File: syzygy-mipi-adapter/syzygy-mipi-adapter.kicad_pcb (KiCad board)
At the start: 4 copper layers, 45 x 70 mm, 67 parts, among them J1 Conn_02x06_Odd_Even, J10 501951-2230, J2 SYZYGY_STD, J3 Conn_01x02, J5 SM03B-SRSS-TB, J8 501951-2230, J9 501951-2230, Q1 DMG1024UV-7, Q2 DMG1024UV-7, U1 RP2350_80QFN, U10 PUSB3F96, U2 W25X20CLSNIG, U3 PUSB3F96, U4 PUSB3F96, U5 PUSB3F96, U6 PUSB3F96, U7 PUSB3F96, U8 PUSB3F96, U9 PUSB3F96, Y1 ABM8-272-T3

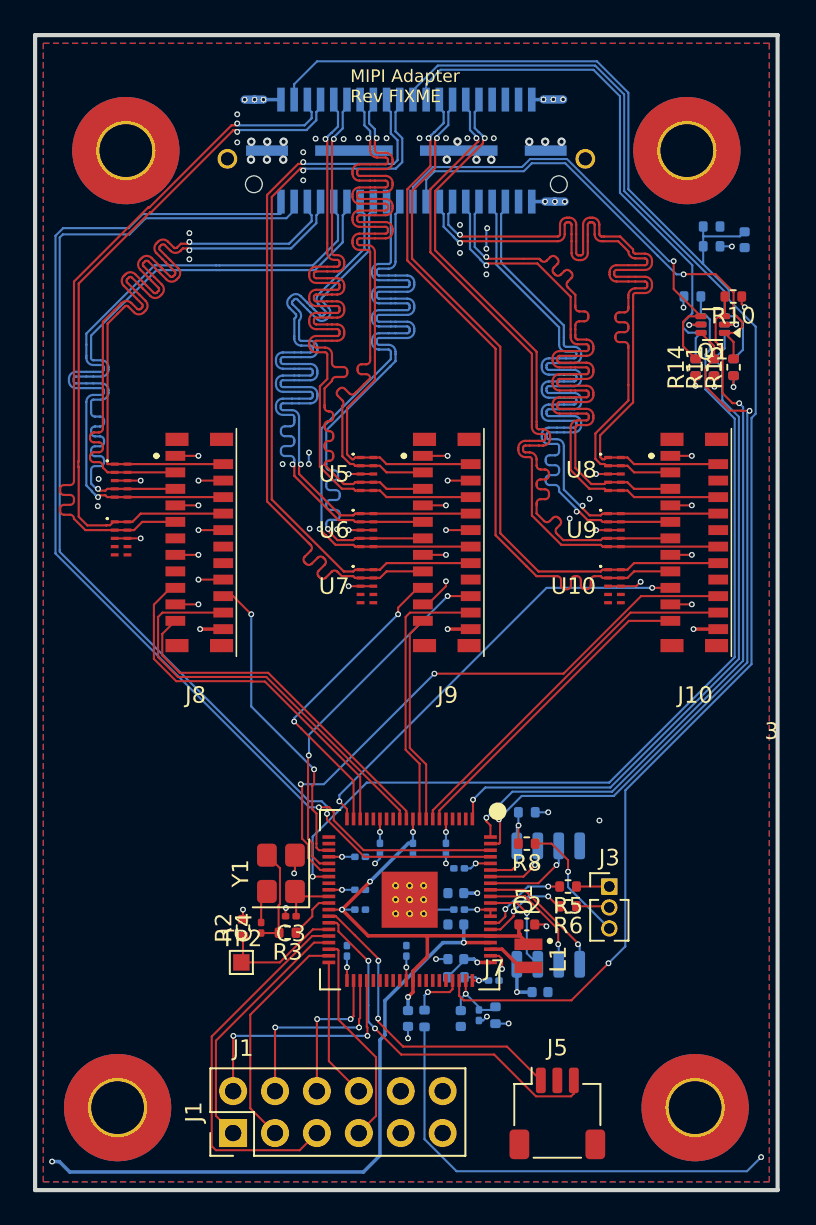
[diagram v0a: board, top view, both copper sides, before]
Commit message: fixes
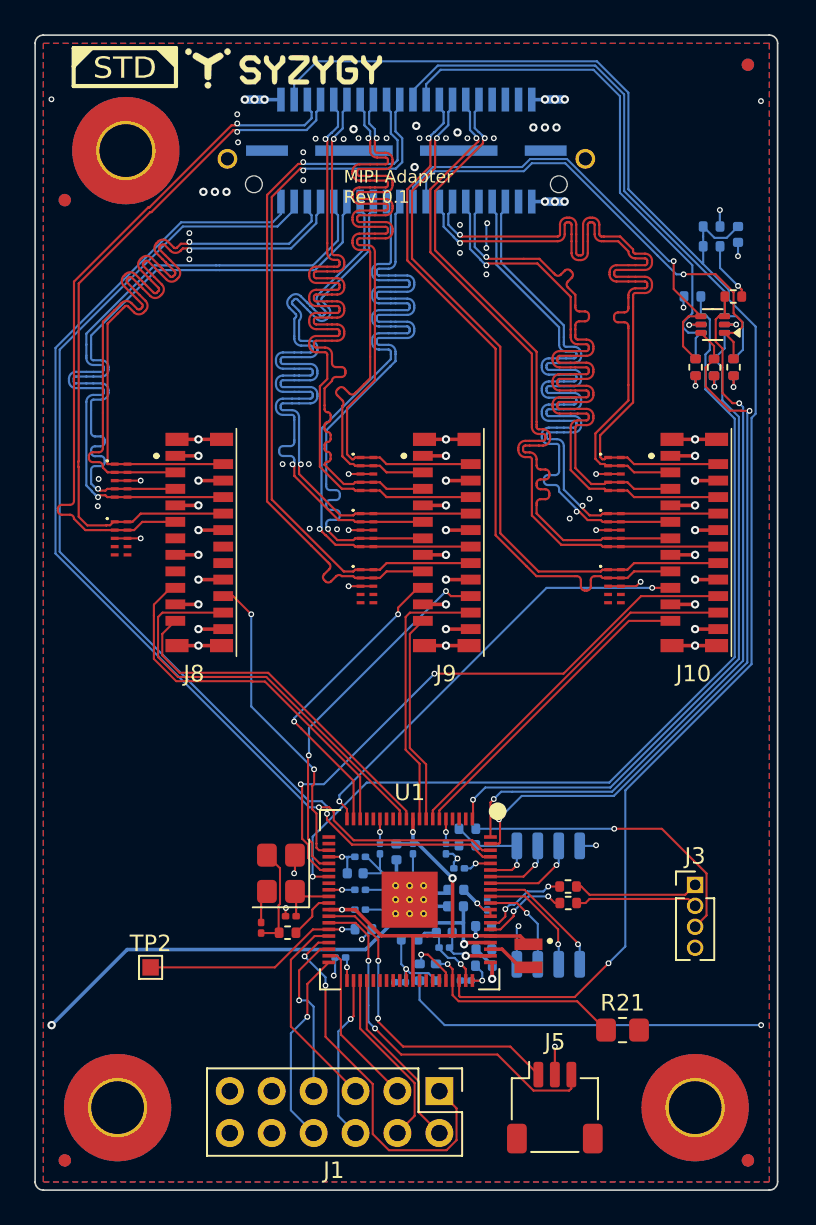
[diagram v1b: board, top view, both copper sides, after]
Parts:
- removed H2: MountingHole_Pad, SYZYGY:MountingHole_3.2mm_M3_6.5mm_Pad_TopBottom
- added FID1: Fiducial, Fiducial:Fiducial_0.75mm_Mask1.5mm, F.Cu at (101.8, 70.0)
- added FID2: Fiducial, Fiducial:Fiducial_0.75mm_Mask1.5mm, F.Cu at (143.2, 61.8)
- added FID3: Fiducial, Fiducial:Fiducial_0.75mm_Mask1.5mm, F.Cu at (101.8, 128.2)
- added FID4: Fiducial, Fiducial:Fiducial_0.75mm_Mask1.5mm, F.Cu at (143.2, 128.2)
- added FID5: Fiducial, Fiducial:Fiducial_0.75mm_Mask1.5mm, B.Cu at (101.8, 70.0)
- added FID6: Fiducial, Fiducial:Fiducial_0.75mm_Mask1.5mm, B.Cu at (143.2, 61.8)
- added FID7: Fiducial, Fiducial:Fiducial_0.75mm_Mask1.5mm, B.Cu at (101.8, 128.2)
- added FID8: Fiducial, Fiducial:Fiducial_0.75mm_Mask1.5mm, B.Cu at (143.2, 128.2)
- added LOGO1: SYZYGY STD logo, SYZYGY:SYZYGY_STD_Logo, F.Cu at (108.5, 63.1)
- added LOGO2: SYZYGY logo, SYZYGY:SYZYGY_Logo, F.Cu at (115.0, 62.0)
- added R20: 10K, Resistor_SMD:R_0402_1005Metric, B.Cu at (124.3, 116.8)
- added R21: 0805, Resistor_SMD:R_0805_2012Metric_Pad1.20x1.40mm_HandSolder, F.Cu at (135.6, 120.3)
- C2, R2, R8: moved to B.Cu
- J3: footprint Connector_PinHeader_1.27mm:PinHeader_1x03_P1.27mm_Vertical -> Connector_PinHeader_1.27mm:PinHeader_1x04_P1.27mm_Vertical
- U2: value W25X20CLSNIG -> W25Q32JVSSIQ
- moved C33 13.3 mm to (119.4, 110.8)
- moved J1 12.8 mm to (124.5, 124.0), turned to -90 degrees
- moved C8 10.1 mm to (121.9, 109.5)
- moved R2 7.30 mm to (119.9, 114.2), turned to 0 degrees
- moved R4 6.94 mm to (122.7, 114.8), turned to 0 degrees
- moved TP2 5.51 mm to (107.0, 116.5)
- moved C38 5.30 mm to (124.8, 114.4), turned to 0 degrees
- moved J3 5.20 mm to (140.0, 111.5)
- moved C35 4.61 mm to (124.8, 115.3), turned to 0 degrees
- moved R9 4.12 mm to (126.2, 109.1), turned to 180 degrees
- moved R8 3.71 mm to (126.2, 108.1)
- moved R7 2.82 mm to (123.3, 116.8)
- moved C2 2.62 mm to (127.2, 114.0)
- moved C42 1.94 mm to (122.1, 117.4), turned to 180 degrees
- moved R1 1.84 mm to (127.2, 116.4), turned to 180 degrees
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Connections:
- R7 pad 2: Net-(U1-GPIO46_ADC6) -> Net-(U1-GPIO45_ADC5)
- U1 pad 56: unconnected-(U1-GPIO45_ADC5-Pad56) -> Net-(U1-GPIO45_ADC5)
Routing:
- net GND: track 51.5 -> 94.4 mm, vias 76 -> 81
- net /USB_BOOTn: track 7.58 -> 18.6 mm
- net Net-(J1-Pin_5): track 23.2 -> 12.5 mm
- net Net-(U1-GPIO46_ADC6): track 3.27 -> 12.9 mm
- net Net-(J1-Pin_1): track 15.3 -> 23.4 mm, vias 0 -> 2
- net P3V3D: track 30.0 -> 37.5 mm, vias 24 -> 20
- net P5VD: track 54.1 -> 46.7 mm, vias 5 -> 6
- net PVIOD: track 61.8 -> 56.0 mm, vias 8 -> 9
- net Net-(J3-Pin_1): track 1.99 -> 7.65 mm
- net /RESETn: track 7.76 -> 13.3 mm, vias 0 -> 1
- net Net-(J3-Pin_2): track 2.02 -> 7.59 mm
- net /SDA_DNA: track 68.7 -> 64.7 mm
- net /SCL_DNA: track 68.3 -> 64.3 mm
- net Net-(J1-Pin_3): track 14.0 -> 10.2 mm
- net Net-(J1-Pin_2): track 14.9 -> 11.1 mm, vias 2 -> 0
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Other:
- outline, holes or cut-outs redrawn
- board text added: "Carrier board edge"
- board text added: "MIPI Adapter Rev 0.1"
- board text removed: "3"
- board text removed: "J1"
- board text removed: "J7"
- board text removed: "MIPI Adapter Rev FIXME"
